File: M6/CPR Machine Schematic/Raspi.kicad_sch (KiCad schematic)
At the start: 2 parts, among them J3 Raspberry_Pi_2_3

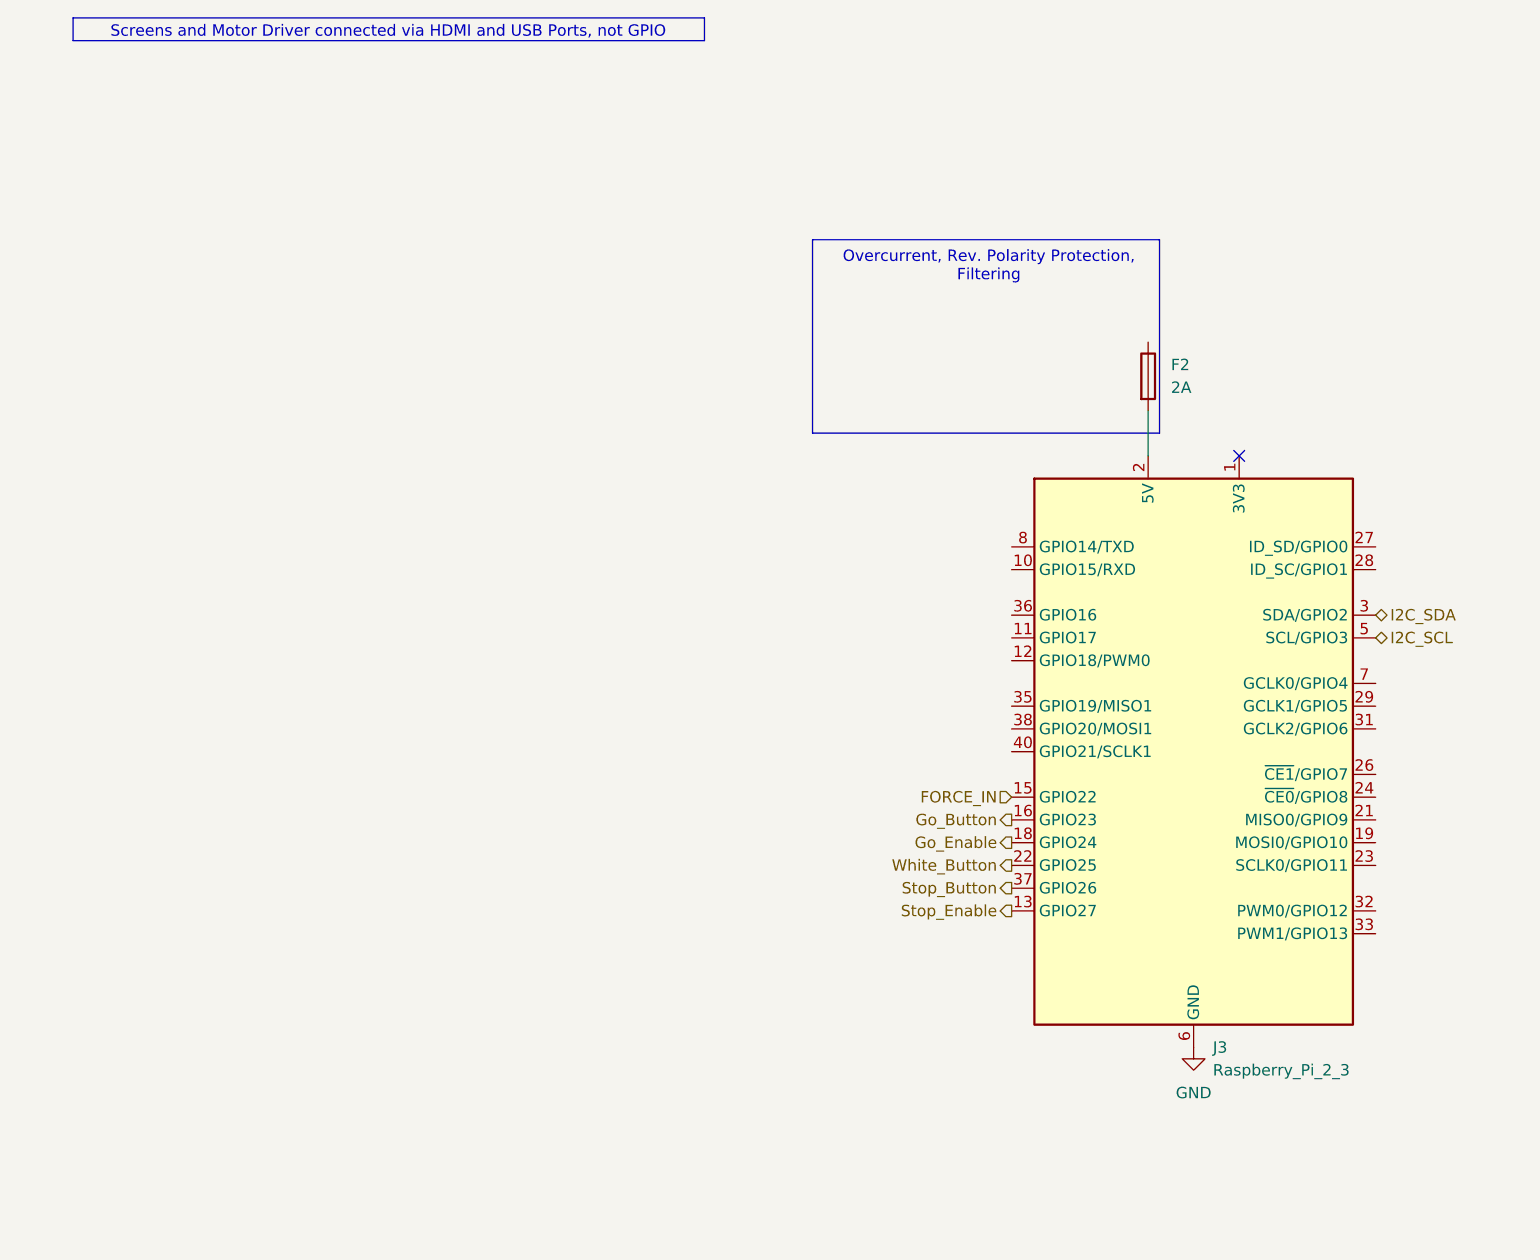
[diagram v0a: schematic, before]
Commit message: More PCB Progress
All Footprints
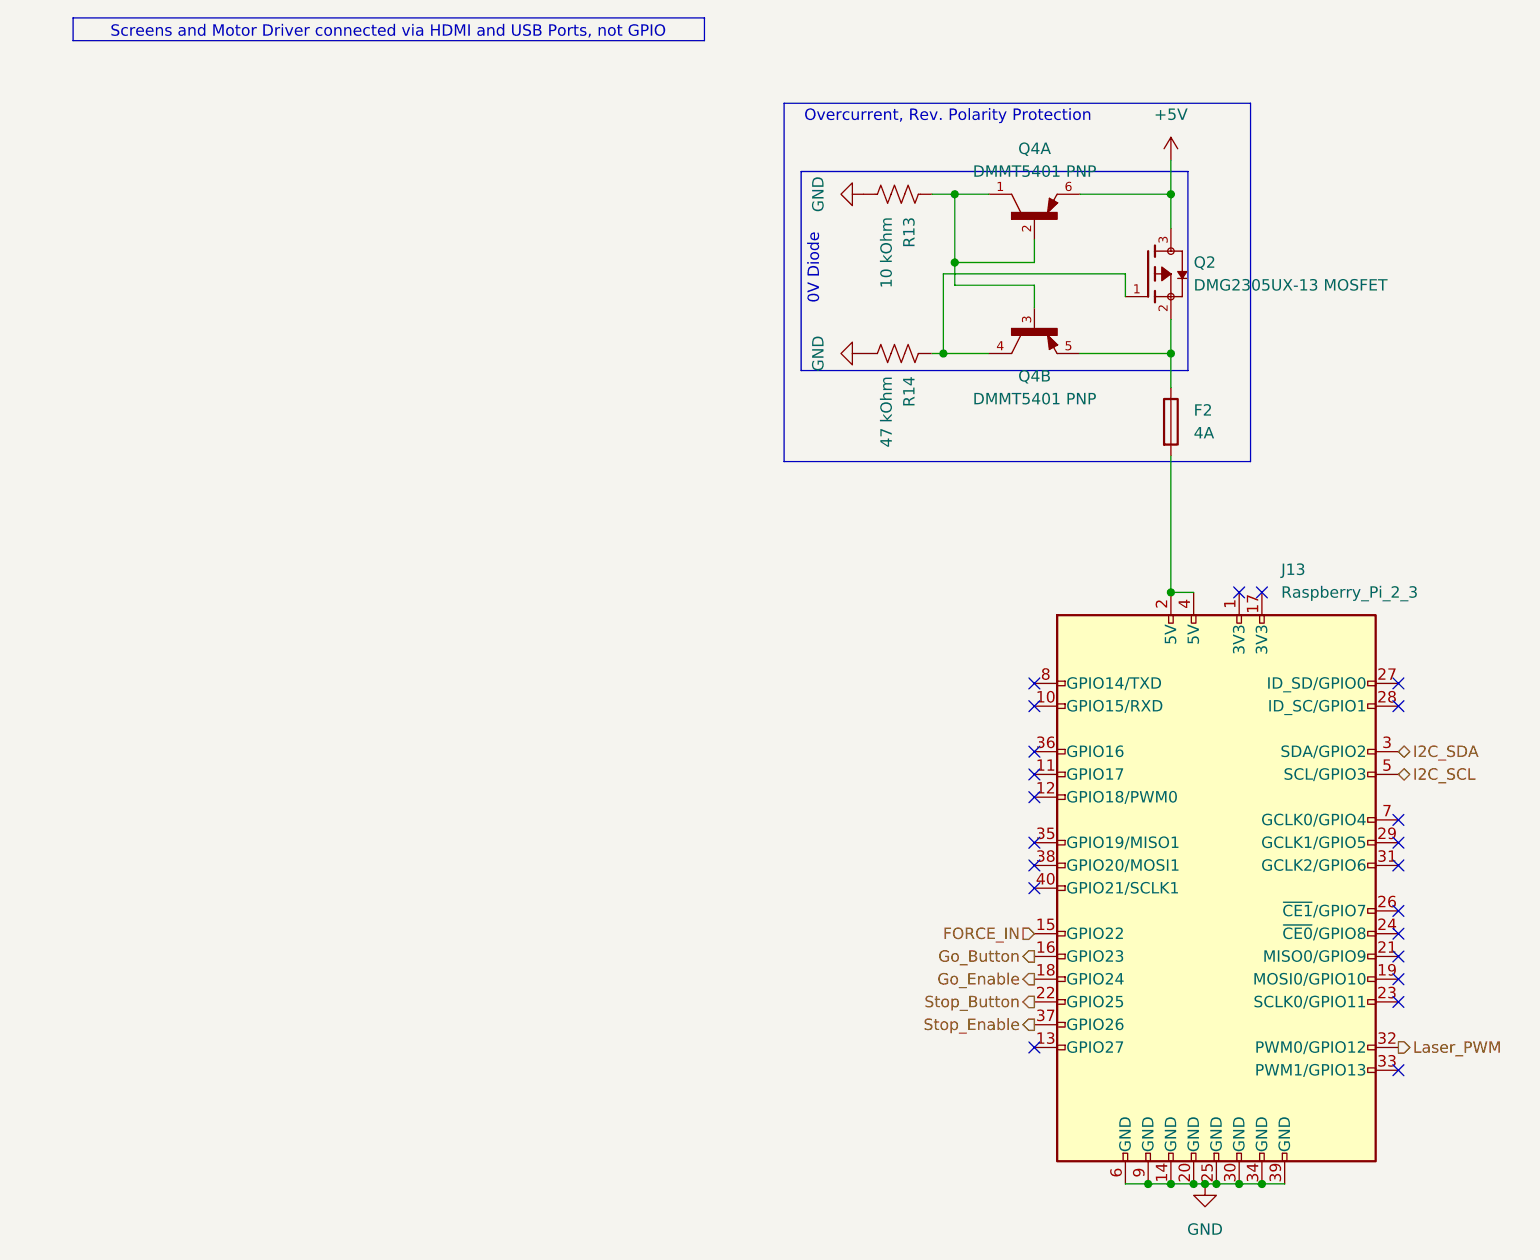
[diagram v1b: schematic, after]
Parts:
- removed J3: Raspberry_Pi_2_3, symbol Connector:Raspberry_Pi_2_3
- added J13: Raspberry_Pi_2_3, Connector_PinSocket_2.54mm:PinSocket_2x20_P2.54mm_Vertical, symbol 2679:Raspberry_Pi_2_3
- added Q2: DMG2305UX-13 MOSFET, 2679:SOT91P240X110-3N, symbol 2679:DMG2305UX-13 MOSFET
- added Q4: DMMT5401 PNP, 2679:SOT95P285X140-6N, symbol 2679:DMMT5401 PNP
- added R13: 10 kOhm, Resistor_SMD:R_1206_3216Metric, symbol Device:R_US
- added R14: 47 kOhm, Resistor_SMD:R_1206_3216Metric, symbol Device:R_US
- F2: value 2A -> 4A; footprint (none) -> Fuse:Fuse_1206_3216Metric
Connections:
- net FORCE_IN: now also J13.15 (GPIO22)
- net GND: now also J13.14 (GND), J13.20 (GND), J13.25 (GND), J13.30 (GND), J13.34 (GND), J13.39 (GND), J13.6 (GND), J13.9 (GND), R13.2, R14.2
- net Go_Button: now also J13.16 (GPIO23)
- net Go_Enable: now also J13.18 (GPIO24)
- net I2C_SCL: now also J13.5 (SCL/GPIO3)
- net I2C_SDA: now also J13.3 (SDA/GPIO2)
- net Stop_Button: now also J13.22 (GPIO25)
- net Stop_Enable: now also J13.37 (GPIO26)
- net at F2.1: now also Q2.2, Q4.5
- net at F2.2: now also J13.2 (5V), J13.4 (5V)
- new net: Q4.1, Q4.2, Q4.3, R13.1
- new net: Q2.1, Q4.4, R14.1
- new net +5V: Q2.3, Q4.6
- new net Laser_PWM: J13.32 (PWM0/GPIO12)
- no-connect marks 1 -> 22
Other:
- note added: "0V Diode"
- note added: "Overcurrent, Rev. Polarity Protection"
- note removed: "Overcurrent, Rev. Polarity Protection, Filtering"
- moved on the sheet: F2

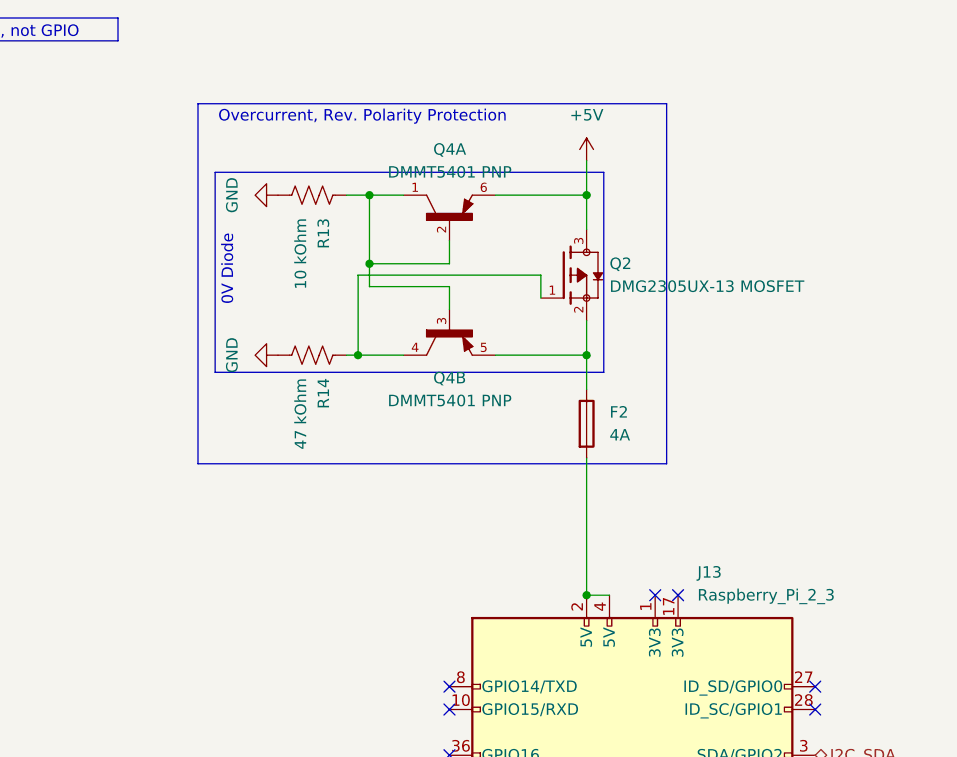
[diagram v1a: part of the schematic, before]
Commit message: finished PCB Draft
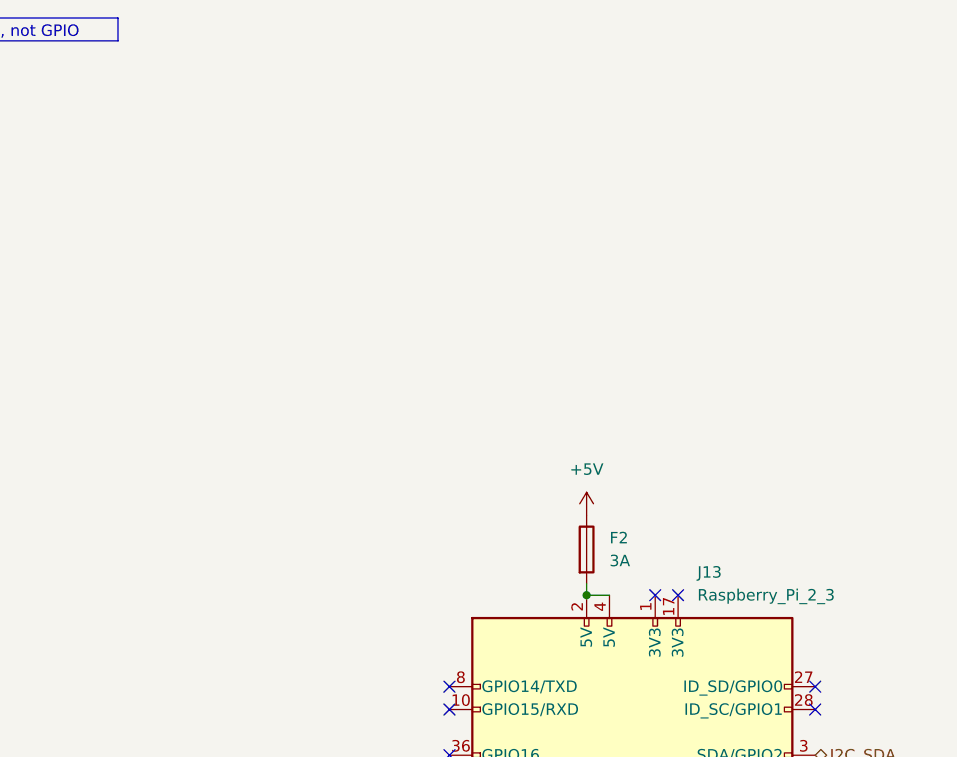
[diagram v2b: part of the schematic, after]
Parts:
- removed Q2: DMG2305UX-13 MOSFET, 2679:SOT91P240X110-3N, symbol 2679:DMG2305UX-13 MOSFET
- removed Q4: DMMT5401 PNP, 2679:SOT95P285X140-6N, symbol 2679:DMMT5401 PNP
- removed R13: 10 kOhm, Resistor_SMD:R_1206_3216Metric, symbol Device:R_US
- removed R14: 47 kOhm, Resistor_SMD:R_1206_3216Metric, symbol Device:R_US
- F2: value 4A -> 3A
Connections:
- net +5V: now also F2.1
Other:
- note removed: "0V Diode"
- note removed: "Overcurrent, Rev. Polarity Protection"
- moved on the sheet: F2
